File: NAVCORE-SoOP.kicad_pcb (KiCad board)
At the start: 6 copper layers, 45 x 46 mm, 148 parts, among them J1 USB-C, J2 ESC 8P, J3 GPS+I2C, J8 microSD, P41 TEL_5V, P42 TEL_TX, P43 TEL_RX, P44 TEL_PPS, P45 TEL_RTS, P46 TEL_GND, P51 RC_5V, P52 RC_TX, P53 RC_RX, P54 RC_GND, P61 CAN_5V, P62 CANH, P63 CANL, P64 CAN_GND, P71 RF_5V, P72 RF_TX, P73 RF_RX, P74 RF_GND, Q1 AO3400A, Q3 AO3400A, SW1 BOOT, SW2 RESET, U1 STM32H743VIT6, U10 TLV75533, U11 SN65HVD230, U12 USBLC6-2SC6, U17 74LVC1G17, U18 TPS54202, U2 ICM-42688-P, U3 ICM-42605, U4 MS5611, U5 W25Q128JVSIQ, U6 PMW3901, U7 VL53L1X, U8 TPS54202, U9 AP2112K-3.3, Y1 8MHz

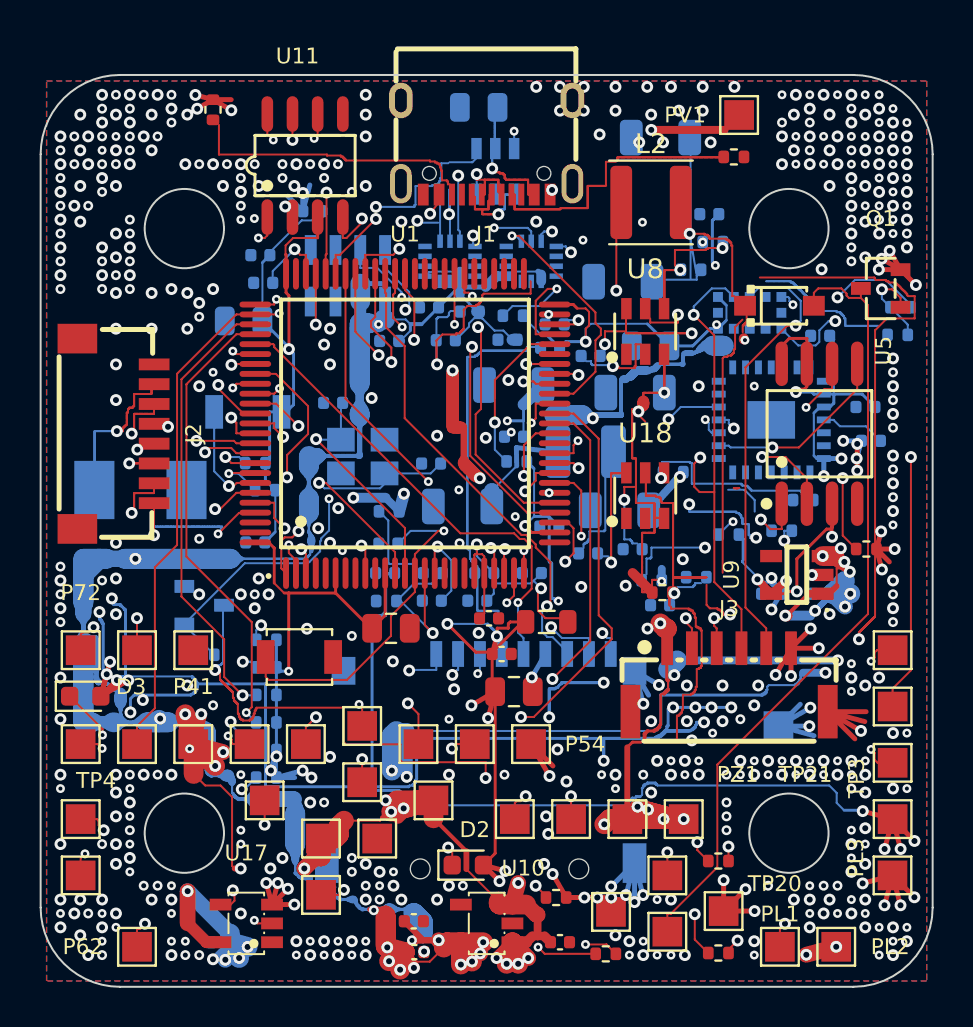
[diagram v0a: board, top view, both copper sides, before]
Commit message: rev B re-layout and re-route
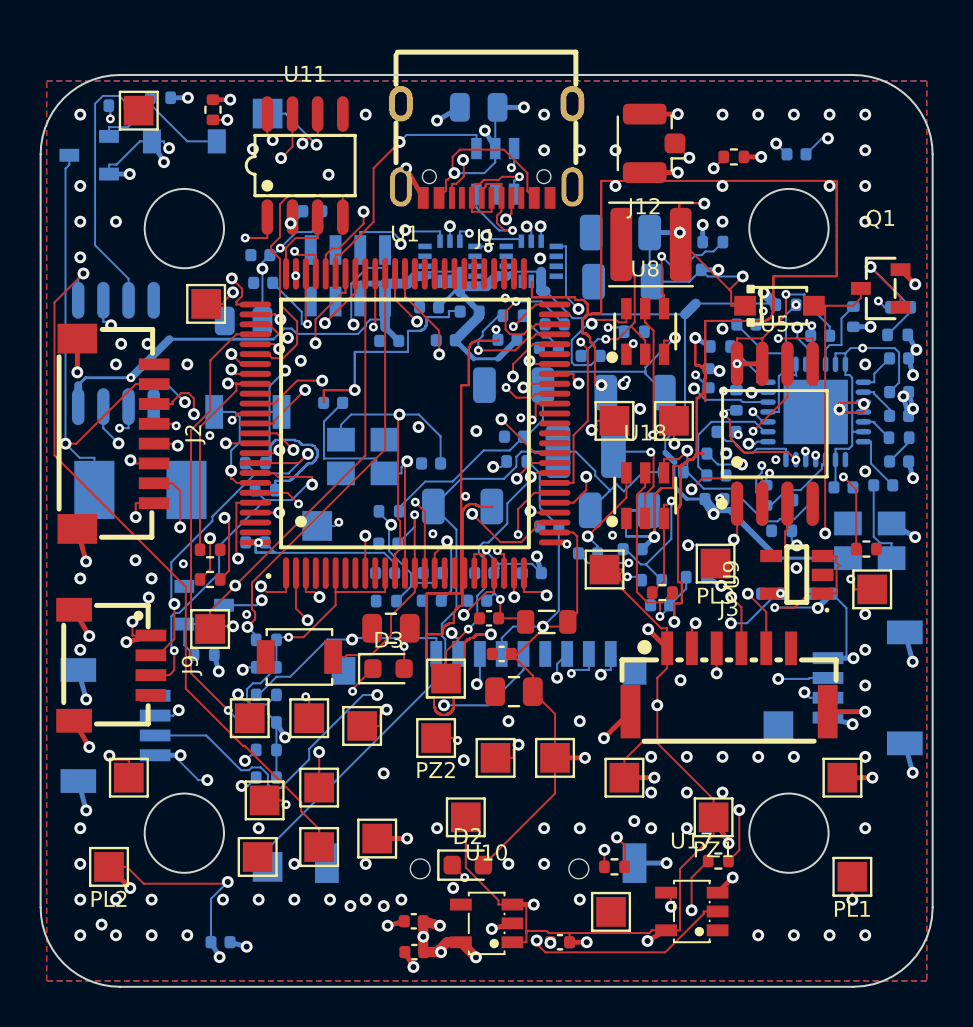
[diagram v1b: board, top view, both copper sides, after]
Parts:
- removed C37, C38, C39: 100n, Capacitor_SMD:C_0402_1005Metric
- removed C40: 4u7, Capacitor_SMD:C_0805_2012Metric
- removed P42: TEL_TX, TestPoint:TestPoint_Pad_1.5x1.5mm
- removed P43: TEL_RX, TestPoint:TestPoint_Pad_1.5x1.5mm
- removed P45: TEL_RTS, TestPoint:TestPoint_Pad_1.5x1.5mm
- removed P51: RC_5V, TestPoint:TestPoint_Pad_1.5x1.5mm
- removed P52: RC_TX, TestPoint:TestPoint_Pad_1.5x1.5mm
- removed P53: RC_RX, TestPoint:TestPoint_Pad_1.5x1.5mm
- removed P54: RC_GND, TestPoint:TestPoint_Pad_1.5x1.5mm
- removed R13: 10k, Resistor_SMD:R_0402_1005Metric
- removed U6: PMW3901, jlc:COB-28_L6.0-W6.0-P0.65-TL-EP
- removed U7: VL53L1X, jlc:OPTO-SMD_VL53L1CXV0FY-1
- added C49: 100n, Capacitor_SMD:C_0402_1005Metric, B.Cu at (135.6, 112.6)
- added C50: 100n, Capacitor_SMD:C_0402_1005Metric, B.Cu at (143.3, 116.0)
- added C51: 1u, Capacitor_SMD:C_0402_1005Metric, B.Cu at (140.5, 120.8)
- added C52: 100p, Capacitor_SMD:C_0402_1005Metric, B.Cu at (138.1, 104.0)
- added C56: 10n, Capacitor_SMD:C_0402_1005Metric, B.Cu at (143.3, 117.2)
- added C57: 10n, Capacitor_SMD:C_0402_1005Metric, B.Cu at (143.3, 119.5)
- added C58: 1n, Capacitor_SMD:C_0402_1005Metric, B.Cu at (142.5, 120.7)
- added C59: 100n, Capacitor_SMD:C_0402_1005Metric, B.Cu at (134.0, 121.4)
- added C60: 100n, Capacitor_SMD:C_0402_1005Metric, B.Cu at (143.3, 114.3)
- added C61: 100n, Capacitor_SMD:C_0402_1005Metric, B.Cu at (134.6, 118.0)
- added C62: 100n, Capacitor_SMD:C_0402_1005Metric, B.Cu at (134.1, 119.1)
- added C63: 100n, Capacitor_SMD:C_0402_1005Metric, B.Cu at (134.1, 120.2)
- added C64: 100n, Capacitor_SMD:C_0402_1005Metric, B.Cu at (133.7, 115.3)
- added DZ1: BZT52C15, jlc:SOD-123_L2.7-W1.6-LS3.7-RD, B.Cu at (107.2, 103.3)
- added J11: SERIAL2 4P, jlc:CONN-SMD_4P-P1.00_SM04B-SRSS-TB-LF-SN, B.Cu at (103.8, 132.8)
- added J12: U.FL ANT, Connector_Coaxial:U.FL_Hirose_U.FL-R-SMT-1_Vertical, F.Cu at (130.9, 103.5)
- added J5: RC IN, jlc:CONN-SMD_4P-P1.00_SM04B-SRSS-TB-LF-SN, B.Cu at (141.7, 130.9)
- added J9: I2C 4P, jlc:CONN-SMD_4P-P1.00_SM04B-SRSS-TB-LF-SN, F.Cu at (103.6, 129.8)
- added Q4: WST4041, jlc:SOT-23-3_L2.9-W1.3-P1.90-LS2.4-BR, B.Cu at (102.5, 104.0)
- added R28: 0R, Resistor_SMD:R_0402_1005Metric, B.Cu at (137.6, 111.6)
- added R29: 0R, Resistor_SMD:R_0402_1005Metric, B.Cu at (134.3, 113.7)
- added R30: 10k, Resistor_SMD:R_0402_1005Metric, B.Cu at (136.6, 121.2)
- added R31: 10k, Resistor_SMD:R_0402_1005Metric, B.Cu at (129.9, 113.0)
- added R34: 1k, Resistor_SMD:R_0402_1005Metric, B.Cu at (143.3, 118.3)
- added R35: 1k, Resistor_SMD:R_0402_1005Metric, B.Cu at (141.0, 112.2)
- added R36: 4k7, Resistor_SMD:R_0402_1005Metric, B.Cu at (104.0, 101.5)
- added R37: 4k7, Resistor_SMD:R_0402_1005Metric, B.Cu at (135.1, 116.4)
- added R46: 100k, Resistor_SMD:R_0402_1005Metric, B.Cu at (106.0, 101.2)
- added TP22: VSERVO, TestPoint:TestPoint_Pad_1.5x1.5mm, F.Cu at (105.0, 101.8)
- added U13: MAX2112, TQFN-28_L5.0-W5.0-P0.50-BL-EP3.3, B.Cu at (139.1, 117.0)
- added U14: OPA2374, jlc:SOP-8_L4.9-W3.9-P1.27-LS6.0-BL, B.Cu at (103.8, 114.0)
- added Y2: 25MHz TCXO, jlc:OSC-SMD_4P-L3.2-W2.5-BL, B.Cu at (141.8, 123.5)
- C1, C10, C11, C12, C13, C14, C15, C16, C19, C2, C21, C26, C27, C28, C29, C3, C30, C31, C32, C33, C34, C35, C36, C4, C41, C43, C44, C46, C5, C65, C66, C68, C73, C8, C9: footprint Capacitor_SMD:C_0402_1005Metric -> C_0402_1005Metric
- C17, C18, C22, C23, C69, C70: footprint Capacitor_SMD:C_1206_3216Metric -> C_1206_3216Metric
- C42, C45, C6, C7: footprint Capacitor_SMD:C_0805_2012Metric -> C_0805_2012Metric
- D1: footprint jlc:DO-214AA_L4.4-W3.6-LS5.3-RD -> DO-214AA_L4.4-W3.6-LS5.3-RD
- D4: footprint jlc:SOD-123F_L2.7-W1.6-LS3.8-RD -> SOD-123F_L2.7-W1.6-LS3.8-RD
- L1: footprint Inductor_SMD:L_0805_2012Metric -> L_0805_2012Metric
- L5: footprint Inductor_SMD:L_1210_3225Metric -> L_1210_3225Metric
- PV1, TP5, TP6: moved to B.Cu
- R10, R11, R12, R18, R19, R38, R39, R4, R40, R41, R42, R43, R5, R6, R7, R9: footprint Resistor_SMD:R_0402_1005Metric -> R_0402_1005Metric
- SW1, SW2: footprint Button_Switch_SMD:SW_SPST_B3U-1000P -> SW_SPST_B3U-1000P
- U12: footprint jlc:SOT-23-6_L2.9-W1.6-P0.95-LS2.8-BL -> SOT-23-6_L2.9-W1.6-P0.95-LS2.8-BL
- U18, U8: footprint SOT-23-6_L2.9-W1.6-P0.95-LS2.8-BL -> jlc:SOT-23-6_L2.9-W1.6-P0.95-LS2.8-BL
- moved PV1 44.8 mm to (111.5, 139.9)
- moved TP4 41.6 mm to (141.9, 126.0)
- moved TP1 38.8 mm to (108.3, 111.5)
- moved TP2 38.7 mm to (104.5, 135.4)
- moved TP5 37.7 mm to (111.5, 102.0), turned to 180 degrees
- moved P63 37.7 mm to (131.9, 117.5)
- moved PL2 36.9 mm to (103.5, 139.9), turned to 180 degrees
- moved P62 35.8 mm to (128.9, 117.5)
- moved R15 27.5 mm to (108.5, 125.5)
- moved R14 24.7 mm to (108.5, 124.0)
- moved P41 22.5 mm to (128.4, 125.0), turned to 180 degrees
- moved U17 22.5 mm to (132.8, 142.2)
- moved TP3 20.0 mm to (123.0, 134.4)
- moved TP6 19.6 mm to (114.0, 122.8), turned to 180 degrees
- moved PL3 18.1 mm to (134.1, 124.7), turned to 180 degrees
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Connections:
- D1 pad 2: VBAT -> VBAT_IN
- J2 pad 2: VBAT -> VBAT_IN
- U1 pad 57: TOF_INT -> (no net)
- U1 pad 58: TOF_XSHUT -> (no net)
- U1 pad 85: EXT_CS1 -> (no net)
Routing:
- net +3V3: track 453.4 -> 119.5 mm, vias 46 -> 14
- net +5V: track 245.7 -> 170.2 mm, vias 46 -> 21
- net +3V3A: track 183.2 -> 124.8 mm, vias 14 -> 7
- net QOUT_N: track 0.00 -> 49.6 mm, vias 0 -> 4
- net IOUT_P: track 0.00 -> 45.9 mm, vias 0 -> 3
- net SOOP_I_ADC: track 35.0 -> 76.1 mm, vias 3 -> 2
- net SWDIO: track 48.7 -> 7.73 mm
- net +9V: track 79.1 -> 38.8 mm, vias 5 -> 0
- net TOF_XSHUT: track 40.3 -> 0.00 mm, vias 3 -> 0
- net QOUT_P: track 0.00 -> 40.1 mm, vias 0 -> 2
- net OPA_IN1N: track 0.00 -> 35.1 mm, vias 0 -> 2
- net UART7_TX: track 33.9 -> 0.00 mm, vias 2 -> 0
- net VCC_RF: track 0.00 -> 33.3 mm, vias 0 -> 2
- net UART7_RTS: track 29.4 -> 0.00 mm, vias 2 -> 0
- net CANH: track 74.8 -> 46.8 mm, vias 3 -> 4
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- removed copper zone on In4.Cu, net +9V
